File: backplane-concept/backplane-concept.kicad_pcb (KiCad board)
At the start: 2 copper layers, 60 x 91.8 mm, 2 parts

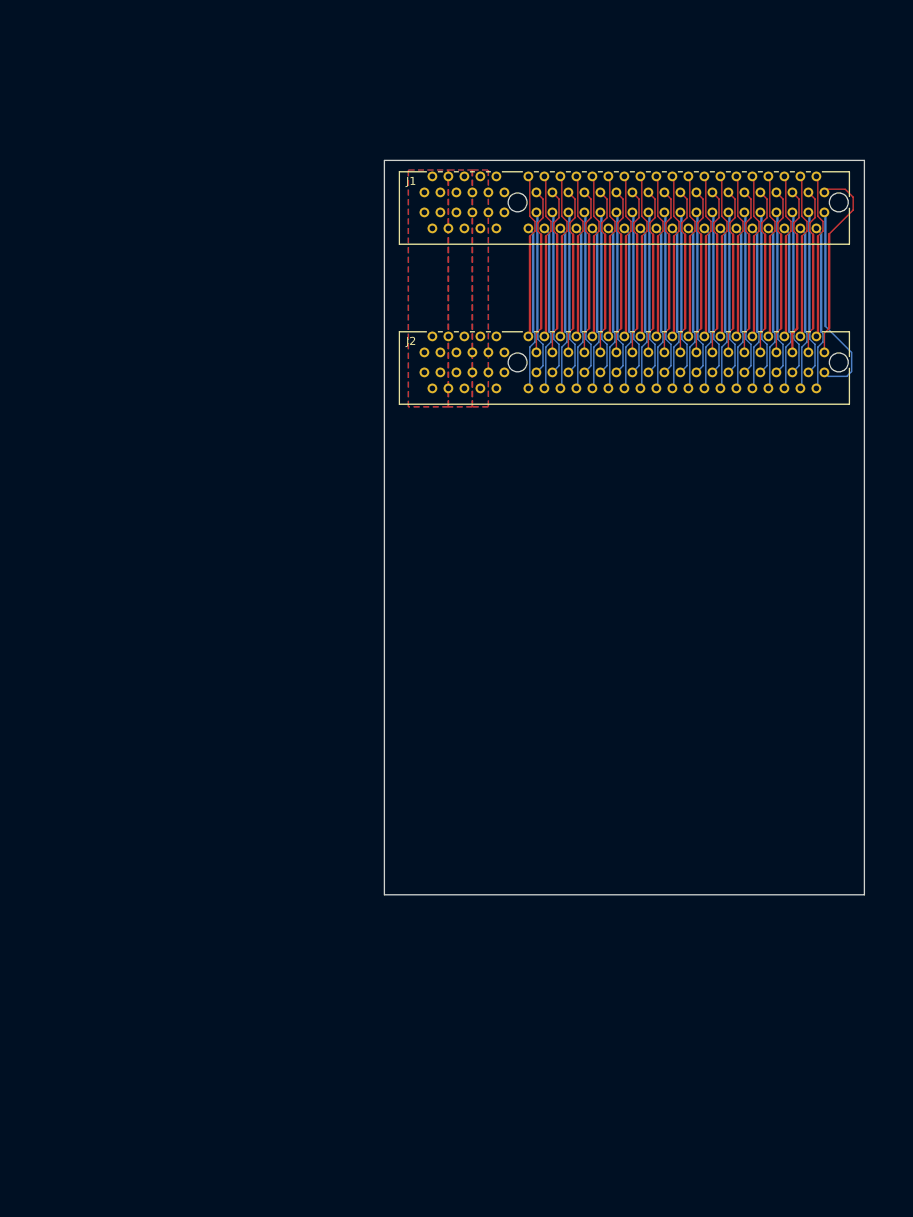
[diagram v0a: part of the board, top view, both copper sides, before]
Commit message: Backplane Ideas
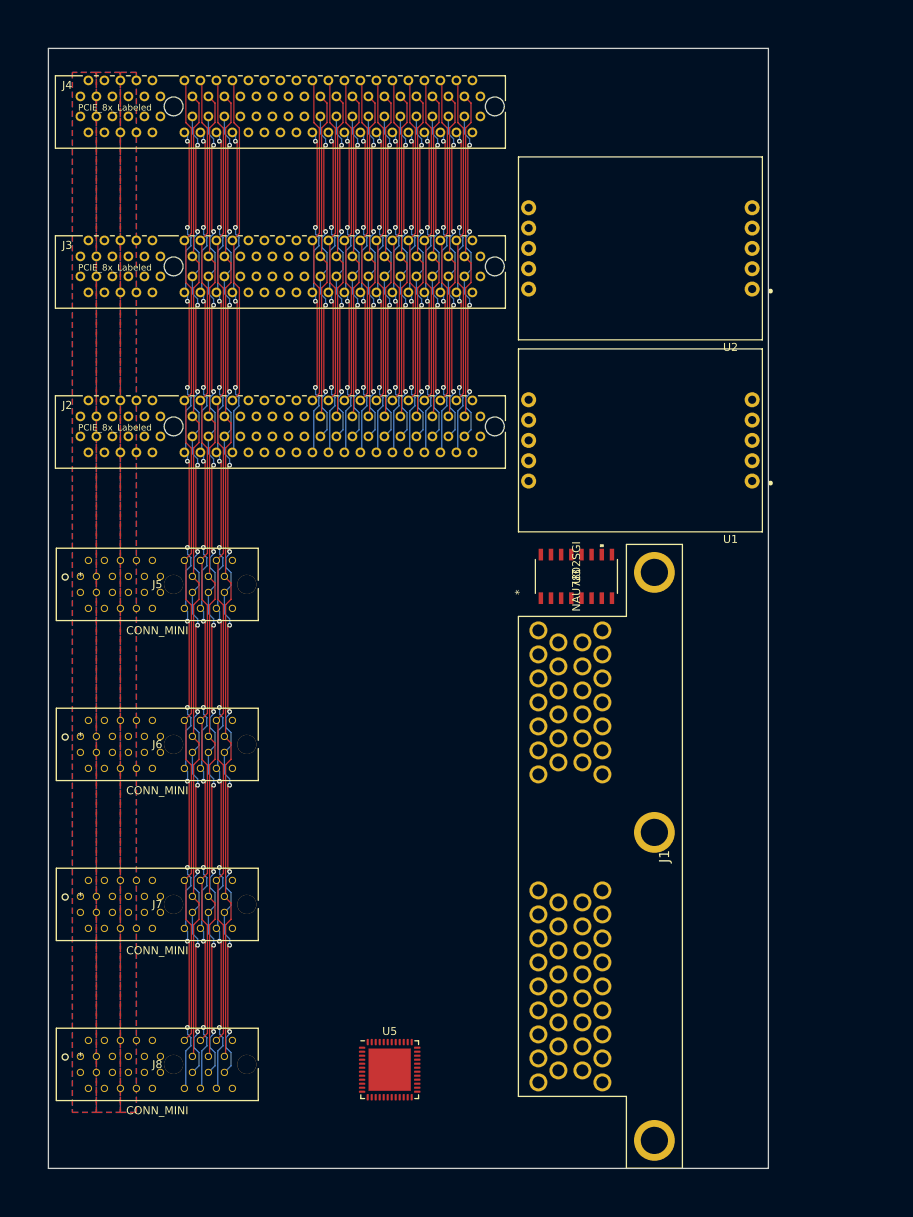
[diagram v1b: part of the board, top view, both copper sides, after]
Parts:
- added J3: PCIE_8x_Labeled, !footprints:9-1734774-5, F.Cu at (60.0, 60.0)
- added J4: PCIE_8x_Labeled, !footprints:9-1734774-5, F.Cu at (60.0, 40.0)
- added J5: CONN_MINI, !footprints:10018784-10200TLF, F.Cu at (60.0, 100.0)
- added J6: CONN_MINI, !footprints:10018784-10200TLF, F.Cu at (60.0, 120.0)
- added J7: CONN_MINI, !footprints:10018784-10200TLF, F.Cu at (60.0, 140.0)
- added J8: CONN_MINI, !footprints:10018784-10200TLF, F.Cu at (60.0, 160.0)
- added U1: PRIMARY, !footprints:SPARKFUN_SEN-13879, F.Cu at (130.0, 83.0)
- added U2: SECONDARY, !footprints:SPARKFUN_SEN-13879, F.Cu at (130.0, 59.0)
- added U3: NAU7802SGI, !footprints:NAU7802SGI, F.Cu at (122.0, 100.0)
- added U5: ESP32-PICO-D4, Package_DFN_QFN:QFN-48-1EP_7x7mm_P0.5mm_EP5.3x5.3mm, F.Cu at (98.7, 161.7)
- J1: value ~ -> 6473427-1; footprint !footprints:9-1734774-5 -> !footprints:64734271
- J2: value ~ -> PCIE_8x_Labeled
- moved J1 112.2 mm to (117.2, 163.2), turned to 90 degrees
- moved J2 43.7 mm to (60.0, 80.0)
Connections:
- J1 pad A1: 5V -> +5V
- J1 pad A10: GND -> +5V
- J1 pad A11: GND -> ENCA_P
- J1 pad A12: ENGHALL1 -> ~ENCA_P
- J1 pad A13: DIR2 -> ENCB_P
- J1 pad A14: DIR1 -> ~ENCB_P
- J1 pad A15: PWM2 -> ENCI_P
- J1 pad A16: PWM1 -> ~ENCI_P
- J1 pad A18: SPARK -> +5V
- J1 pad A19: RRHALL -> ENCA_S
- J1 pad A2: 5V -> HALL1_P
- J1 pad A20: ENGHALL2 -> ~ENCA_S
- J1 pad A21: GND -> ENCB_S
- J1 pad A22: PLOADC1 -> ~ENCB_S
- J1 pad A23: PLOADC2 -> ENCI_S
- J1 pad A24: PLDCLK -> ~ENCI_S
- J1 pad A25: PLDDAT -> GND
- J1 pad A26: SLOADC1 -> +5V
- J1 pad A27: SLOADC2 -> HALL1_S
- J1 pad A28: SLDCLK -> HALL2_S
- J1 pad A29: SLDDAT -> HALL3_S
- J1 pad A3: 5V -> HALL2_P
- J1 pad A30: PENC_A -> GND
- J1 pad A31: ~PENC_A -> THERM_S
- J1 pad A32: PENC_B -> MOT1_S
- J1 pad A33: ~PENC_B -> MOT2_S
- J1 pad A34: SENC_A -> MOT3_S
- J1 pad A4: 3.3V -> HALL3_P
- J1 pad A5: 3.3V -> GND
- J1 pad A6: 3.3V -> THERM_P
- J1 pad A7: 8.4V -> MOT1_P
- J1 pad A8: 8.4V -> MOT2_P
- J1 pad A9: GND -> MOT3_P
- J1 pad B1: 5V -> GND
- J1 pad B10: GND -> +3V3
- J1 pad B12: CAN_H -> GND
- J1 pad B13: CAN_L -> THERM_A1_CASE
- J1 pad B14: GND -> THERM_A2_CASE
- J1 pad B15: I2C_DATA -> GND
- J1 pad B16: I2C_CLK -> IN+_P
- J1 pad B17: GND -> IN-_P
- J1 pad B18: TX1 -> AVDD_S
- J1 pad B19: RX1 -> GND
- J1 pad B2: 5V -> GND
- J1 pad B20: TX2 -> IN+_S
- J1 pad B21: RX2 -> IN-_S
- J1 pad B22: TX3 -> AVDD_S
- J1 pad B23: RX3 -> GND
- J1 pad B24: TX4 -> GND
- J1 pad B25: RX4 -> +3V3
- J1 pad B26: TX5 -> +3V3
- J1 pad B3: 5V -> HALL_ENG1
- J1 pad B4: 3.3V -> HALL_ENG2
- J1 pad B5: 3.3V -> +8V
- J1 pad B6: 3.3V -> +8V
- J1 pad B7: 8.4V -> GND
- J1 pad B8: 8.4V -> I2C1_ECVT_EXT_SDA
- J1 pad B9: GND -> I2C1_ECVT_EXT_SCL
- J2 pad A1: 5V -> +5V
- J2 pad A12: ENGHALL1 -> DAQ_TX0_ECVT_RX0
- J2 pad A13: DIR2 -> DAQ_RX0_ECVT_TX0
- J2 pad A14: DIR1 -> DAQ_TX1_DATA
- J2 pad A15: PWM2 -> GND
- J2 pad A16: PWM1 -> I2C1_DAQ_SDA
- J2 pad A17: GND -> I2C1_DAQ_SCL
- J2 pad A18: SPARK -> GND
- J2 pad A19: RRHALL -> unconnected-(J2-PadA19)
- J2 pad A2: 5V -> +5V
- J2 pad A20: ENGHALL2 -> unconnected-(J2-PadA20)
- J2 pad A21: GND -> unconnected-(J2-PadA21)
- J2 pad A22: PLOADC1 -> unconnected-(J2-PadA22)
- J2 pad A23: PLOADC2 -> unconnected-(J2-PadA23)
- J2 pad A24: PLDCLK -> unconnected-(J2-PadA24)
- J2 pad A25: PLDDAT -> unconnected-(J2-PadA25)
- J2 pad A26: SLOADC1 -> unconnected-(J2-PadA26)
- J2 pad A27: SLOADC2 -> unconnected-(J2-PadA27)
- J2 pad A28: SLDCLK -> GND
- J2 pad A29: SLDDAT -> ENCA_P
- J2 pad A3: 5V -> +5V
- J2 pad A30: PENC_A -> ~ENCA_P
- J2 pad A31: ~PENC_A -> ENCB_P
- J2 pad A32: PENC_B -> ~ENCB_P
- J2 pad A33: ~PENC_B -> ENCI_P
- J2 pad A34: SENC_A -> ~ENCI_P
- J2 pad A35: ~SENC_A -> GND
- J2 pad A36: SENC_B -> ENCA_S
- J2 pad A37: ~SENC_B -> ~ENCA_S
- J2 pad A38: GND -> ENCB_S
- J2 pad A39: DIG_OUT -> ~ENCB_S
- J2 pad A4: 3.3V -> +3V3
- J2 pad A40: N_A -> ENCI_S
- J2 pad A41: IR_TEENSY -> ~ENCI_S
- J2 pad A42: IR_AMP -> SPARK
- J2 pad A43: unconnected-(J2-PadA43) -> GND
- J2 pad A44: unconnected-(J2-PadA44) -> THERM_P
- J2 pad A45: GND -> THERM_S
- J2 pad A46: TEMP4 -> THERM_A1_CASE
- J2 pad A47: TEMP3 -> THERM_A2_CASE
- J2 pad A48: TEMP2 -> THERM_A3
- J2 pad A49: TEMP1 -> THERM_A4
- J2 pad A5: 3.3V -> +3V3
- J2 pad A6: 3.3V -> +3V3
- J2 pad A7: 8.4V -> +8V
- J2 pad A8: 8.4V -> +8V
- J2 pad B1: 5V -> +5V
- J2 pad B14: GND -> I2C0_DAQ_SDA
- J2 pad B15: I2C_DATA -> I2C0_DAQ_SCL
- J2 pad B16: I2C_CLK -> I2C0_ECVT_SDA
- J2 pad B17: GND -> I2C0_ECVT_SCL
- J2 pad B18: TX1 -> GND
- J2 pad B19: RX1 -> unconnected-(J2-PadB19)
- J2 pad B2: 5V -> +5V
- J2 pad B20: TX2 -> unconnected-(J2-PadB20)
- J2 pad B21: RX2 -> unconnected-(J2-PadB21)
- J2 pad B22: TX3 -> unconnected-(J2-PadB22)
- J2 pad B23: RX3 -> unconnected-(J2-PadB23)
- J2 pad B24: TX4 -> unconnected-(J2-PadB24)
- J2 pad B25: RX4 -> unconnected-(J2-PadB25)
- J2 pad B26: TX5 -> unconnected-(J2-PadB26)
- J2 pad B27: RX5 -> unconnected-(J2-PadB27)
- J2 pad B28: GND -> LOADC_CLK_P
- J2 pad B29: CIPO -> LOADC_DAT_P
- J2 pad B3: 5V -> +5V
- J2 pad B30: COPI -> LOADC_CLK_P
- J2 pad B31: SCLK -> LOADC_DAT_S
- J2 pad B32: CS1 -> GND
- J2 pad B33: CS2 -> HALL_ENG1
- J2 pad B34: CS3 -> HALL_RW
- J2 pad B35: CS4 -> PWM_P
- J2 pad B36: CS5 -> DIR_P
- J2 pad B37: CS6 -> PWM_S
- J2 pad B38: unconnected-(J2-PadB38) -> DIR_S
- J2 pad B39: unconnected-(J2-PadB39) -> I2C1_ECVT_EXT_SDA
- J2 pad B4: 3.3V -> +3V3
- J2 pad B40: unconnected-(J2-PadB40) -> I2C1_ECVT_EXT_SCL
- J2 pad B41: unconnected-(J2-PadB41) -> HALL_ENG2
- J2 pad B43: FRBPRESS -> GND
- J2 pad B44: RRBPRESS -> BP_FRONT
- J2 pad B45: RPOT1 -> BP_REAR
- J2 pad B46: RPOT2 -> RPOT1
- J2 pad B47: VOLT1 -> RPOT2
- J2 pad B48: VOLT2 -> Net-(J2-PadB48)
- J2 pad B49: VOLT3 -> Net-(J2-PadB49)
- J2 pad B5: 3.3V -> +3V3
- J2 pad B6: 3.3V -> +3V3
- J2 pad B7: 8.4V -> +8V
- J2 pad B8: 8.4V -> +8V
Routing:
- net GND: track 166.5 -> 452.8 mm, vias 0 -> 16
- net I2C0_ECVT_SCL: track 0.00 -> 127.0 mm, vias 0 -> 12
- net I2C0_DAQ_SCL: track 0.00 -> 127.0 mm, vias 0 -> 12
- net I2C0_ECVT_SDA: track 0.00 -> 123.8 mm, vias 0 -> 12
- net I2C0_DAQ_SDA: track 0.00 -> 123.8 mm, vias 0 -> 12
- net DAQ_RX0_ECVT_TX0: track 0.00 -> 122.8 mm
- net I2C1_DAQ_SCL: track 0.00 -> 122.8 mm
- net I2C1_DAQ_SDA: track 0.00 -> 122.7 mm
- net DAQ_TX1_DATA: track 0.00 -> 122.7 mm
- net DAQ_TX0_ECVT_RX0: track 0.00 -> 122.7 mm
- net LOADC_CLK_P: track 0.00 -> 82.5 mm, vias 0 -> 8
- net CAN_L: track 62.0 -> 127.0 mm, vias 0 -> 12
- net CAN_H: track 62.0 -> 123.8 mm, vias 0 -> 12
- net PWM_P: track 0.00 -> 42.5 mm, vias 0 -> 4
- net LOADC_DAT_S: track 0.00 -> 42.5 mm, vias 0 -> 4
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- added copper zone on B.Cu, net +3V3
- added copper zone on F.Cu, net +3V3
- added copper zone on B.Cu, net +5V
- added copper zone on F.Cu, net +5V
- added copper zone on B.Cu, net +8V
- added copper zone on F.Cu, net +8V
- removed copper zone on B.Cu, net 3.3V
- removed copper zone on F.Cu, net 3.3V
- removed copper zone on B.Cu, net 5V
- removed copper zone on F.Cu, net 5V
- removed copper zone on B.Cu, net 8.4V
- removed copper zone on F.Cu, net 8.4V
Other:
- board size 60 x 91.8 mm -> 90 x 140 mm
